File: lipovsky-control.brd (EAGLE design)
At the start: 56.2 x 21 mm, 12 parts, among them U1 ATTINYX4A8MU, U10 CCR20MA_45V, U7 LTV-816S

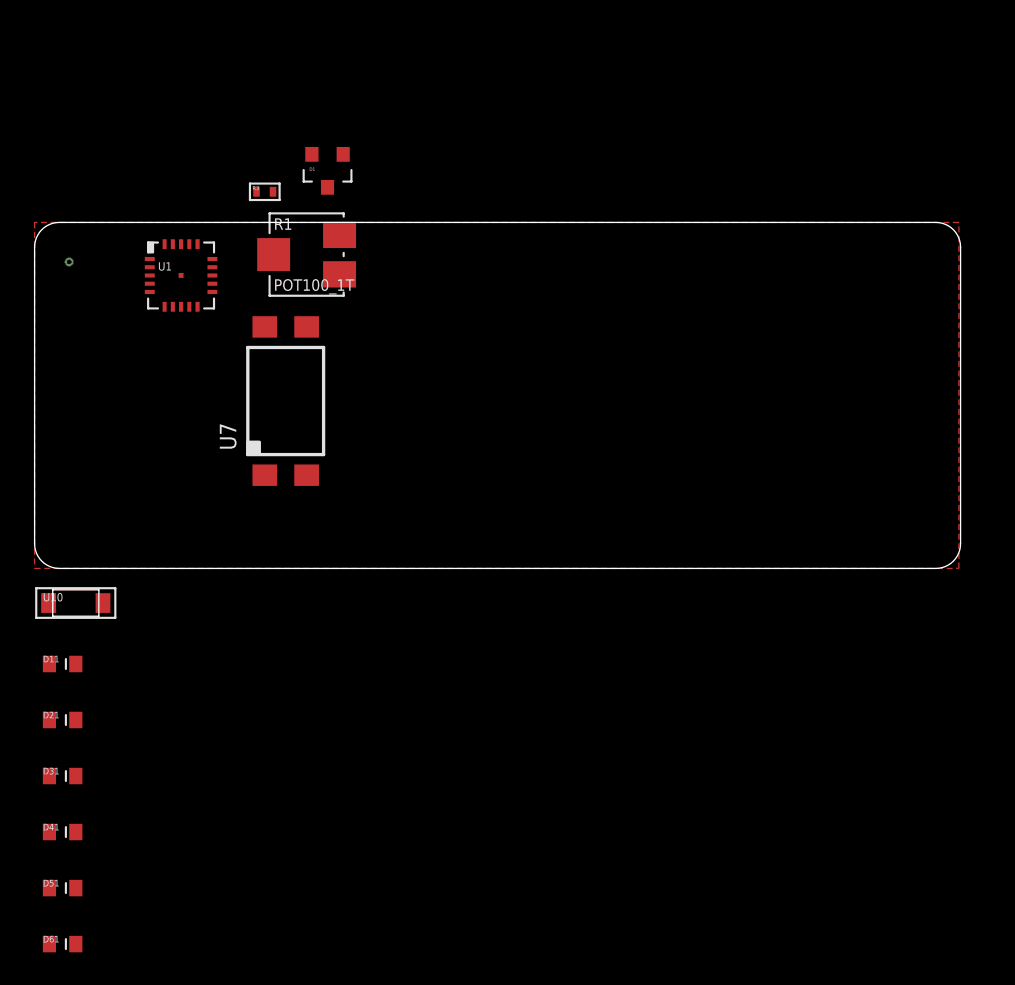
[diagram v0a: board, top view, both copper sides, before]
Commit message: .
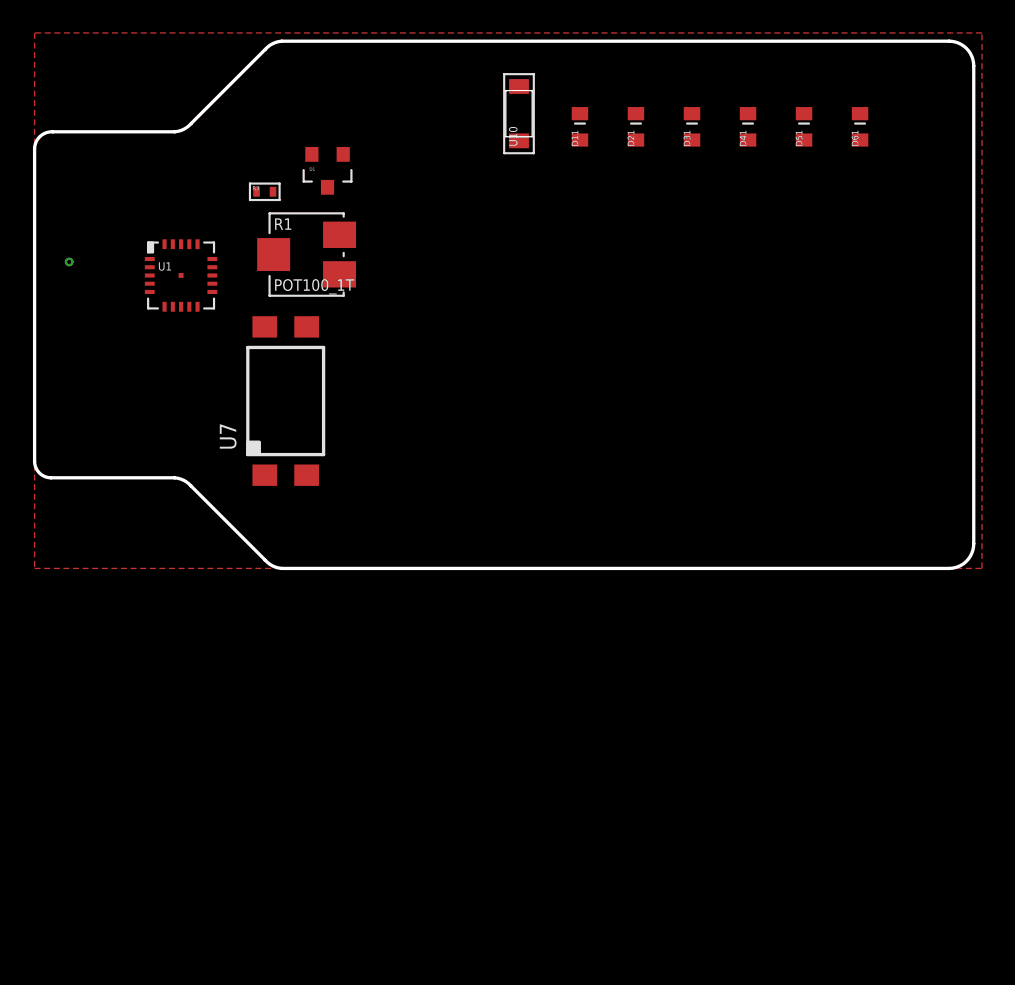
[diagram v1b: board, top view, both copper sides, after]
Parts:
- moved D61 69.3 mm to (50.1, 26.8), turned to 90 degrees
- moved D51 64.5 mm to (46.7, 26.8), turned to 90 degrees
- moved D41 59.7 mm to (43.3, 26.8), turned to 90 degrees
- moved D31 54.9 mm to (39.9, 26.8), turned to 90 degrees
- moved D21 50.1 mm to (36.5, 26.8), turned to 90 degrees
- moved D11 45.3 mm to (33.1, 26.8), turned to 90 degrees
- moved U10 40.1 mm to (29.4, 27.6), turned to 90 degrees
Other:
- board size 56.2 x 21 mm -> 57 x 32 mm
